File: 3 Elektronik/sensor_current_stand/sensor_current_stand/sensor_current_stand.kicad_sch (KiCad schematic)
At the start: 9 parts, among them J1 Conn_01x02_Socket, J2 Conn_01x02_Socket, J3 USB_B, U1 USBLC6-2SC6

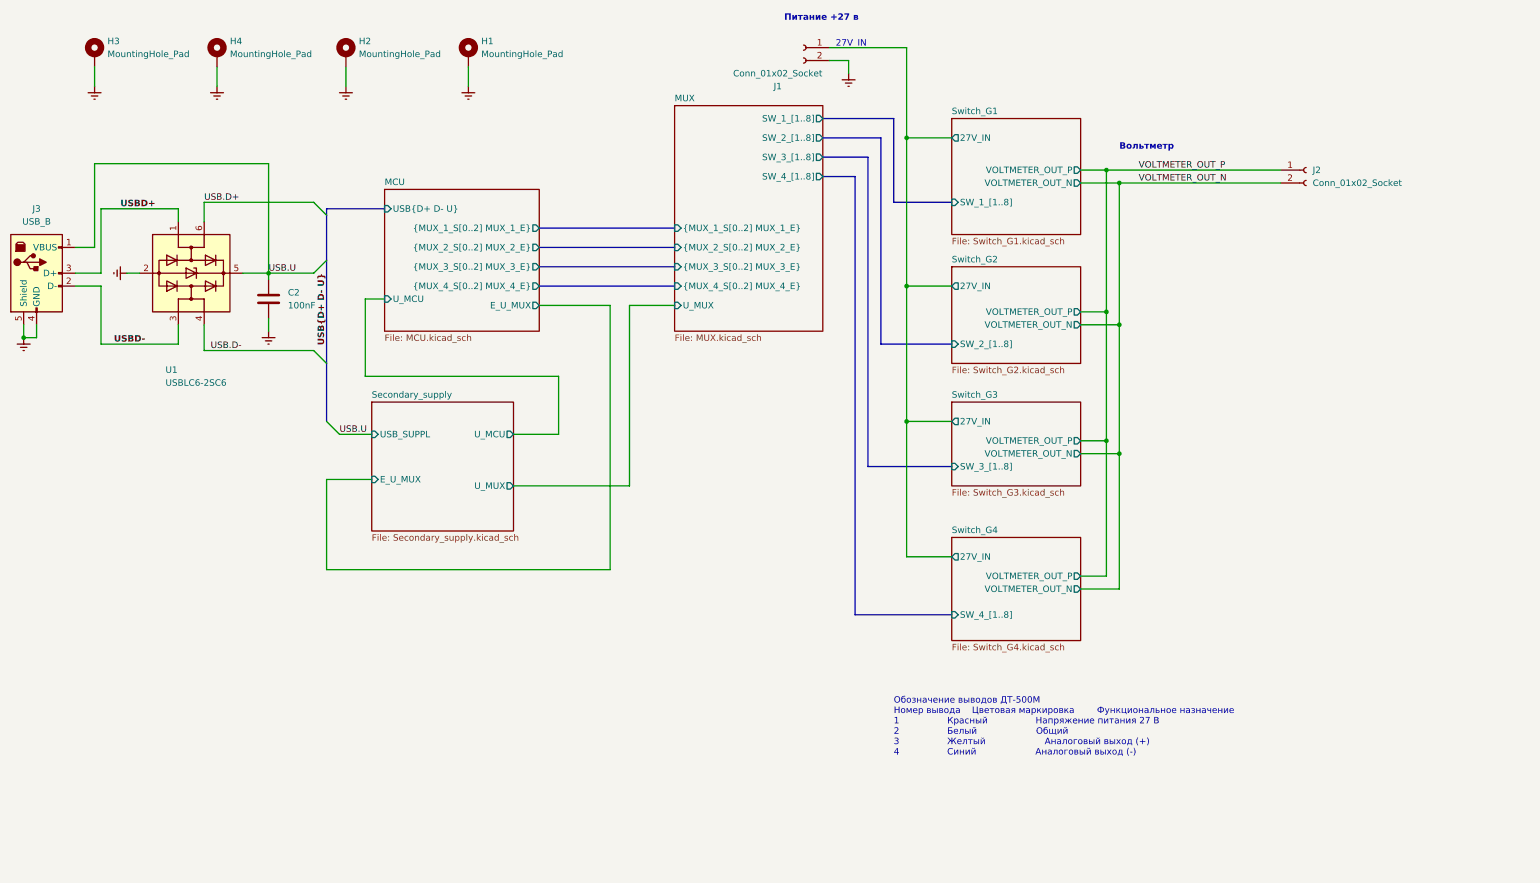
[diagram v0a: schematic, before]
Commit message: Version 2
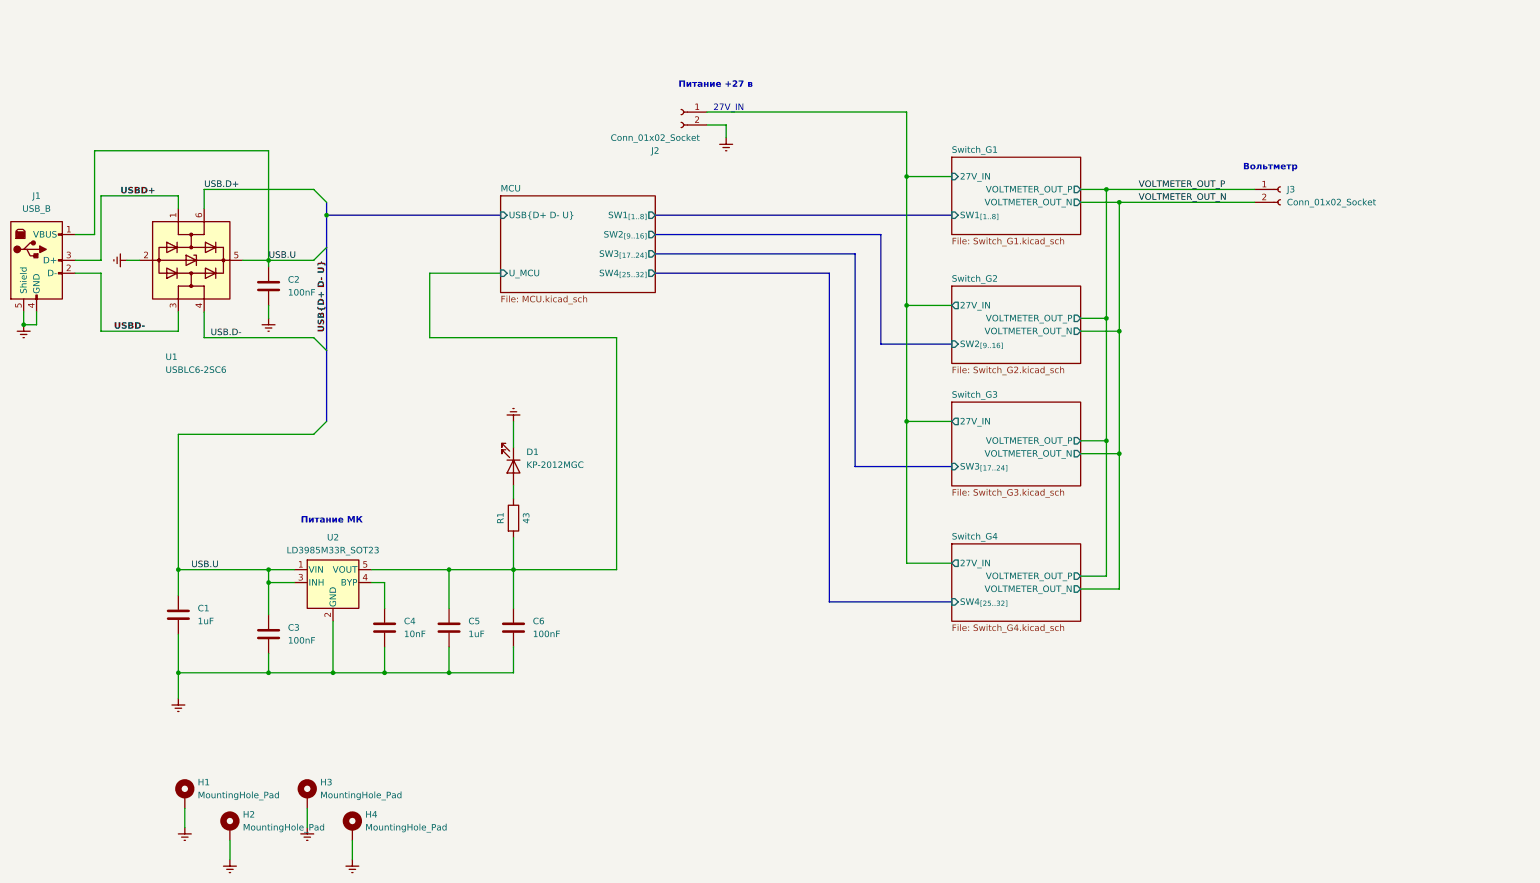
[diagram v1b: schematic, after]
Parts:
- removed H1: MountingHole_Pad, MountingHole:MountingHole_4.3mm_M4_Pad_TopBottom, symbol Mechanical:MountingHole_Pad
- added C1, C5: 1uF, Capacitor_SMD:C_0805_2012Metric, symbol Device:C
- added C3, C6: 100nF, Capacitor_SMD:C_0805_2012Metric, symbol Device:C
- added C4: 10nF, Capacitor_SMD:C_0805_2012Metric, symbol Device:C
- added D1: KP-2012MGC, LED_SMD:LED_0805_2012Metric_Pad1.15x1.40mm_HandSolder, symbol Device:LED
- added H4: MountingHole_Pad, MountingHole:MountingHole_4.3mm_M4_Pad_TopBottom, symbol Mechanical:MountingHole_Pad
- added R1: 43, Resistor_SMD:R_1206_3216Metric_Pad1.30x1.75mm_HandSolder, symbol Device:R
- added U2: LD3985M33R_SOT23, Package_TO_SOT_SMD:SOT-23-5, symbol Regulator_Linear:LD3985M33R_SOT23
- renumbered H3 to H1, H4 to H3, J3 to J1, J1 to J2, J2 to J3
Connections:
- net Earth: now also C1.2, C3.2, C4.2, C5.2, C6.2, D1.1 (K), H4.1, U2.2 (GND)
- net MCU/U_MCU: now also C5.1, C6.1, R1.2, U2.5 (VOUT)
- net USB.U: now also C1.1, C3.1, U2.1 (VIN), U2.3 (INH)
- new net: D1.2 (A), R1.1
- new net: C4.1, U2.4 (BYP)
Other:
- removed sheet MUX
- removed sheet Secondary_supply
- sheet MCU ports: added SW1_{[1..8]}, SW2_{[9..16]}, SW3_{[17..24]}, SW4_{[25..32]}; removed E_U_MUX, {MUX_1_S[0..2] MUX_1_E}, {MUX_2_S[0..2] MUX_2_E}, {MUX_3_S[0..2] MUX_3_E}, {MUX_4_S[0..2] MUX_4_E}
- sheet Switch_G1 ports: added SW1_{[1..8]}; removed SW_1_[1..8]
- sheet Switch_G2 ports: added SW2_{[9..16]}; removed SW_2_[1..8]
- sheet Switch_G3 ports: added SW3_{[17..24]}; removed SW_3_[1..8]
- sheet Switch_G4 ports: added SW4_{[25..32]}; removed SW_4_[1..8]
- note added: "Питание МК"
- note removed: "Обозначение выводов ДТ-500М Номер вывода Цветовая маркировка Функциональное назначение 1 Красный Напряжение питания 27 В 2 Белый Общий 3 Желтый Аналоговый выход (+) 4 Синий Аналоговый выход (-)"
- moved on the sheet: C2, H1, H3, J1, J2, J3, U1
